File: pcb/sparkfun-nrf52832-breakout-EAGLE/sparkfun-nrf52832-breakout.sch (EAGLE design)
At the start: 72 parts, among them J1 DNP, Q1 2.5A/30V, U1 ESP8266, U2 MCP73831, U3 AT25SF041-SOIC8, U4 AP2112K-3.3V, U5 DNP, U6 DNP, U7 DNP, Y1 26MHz

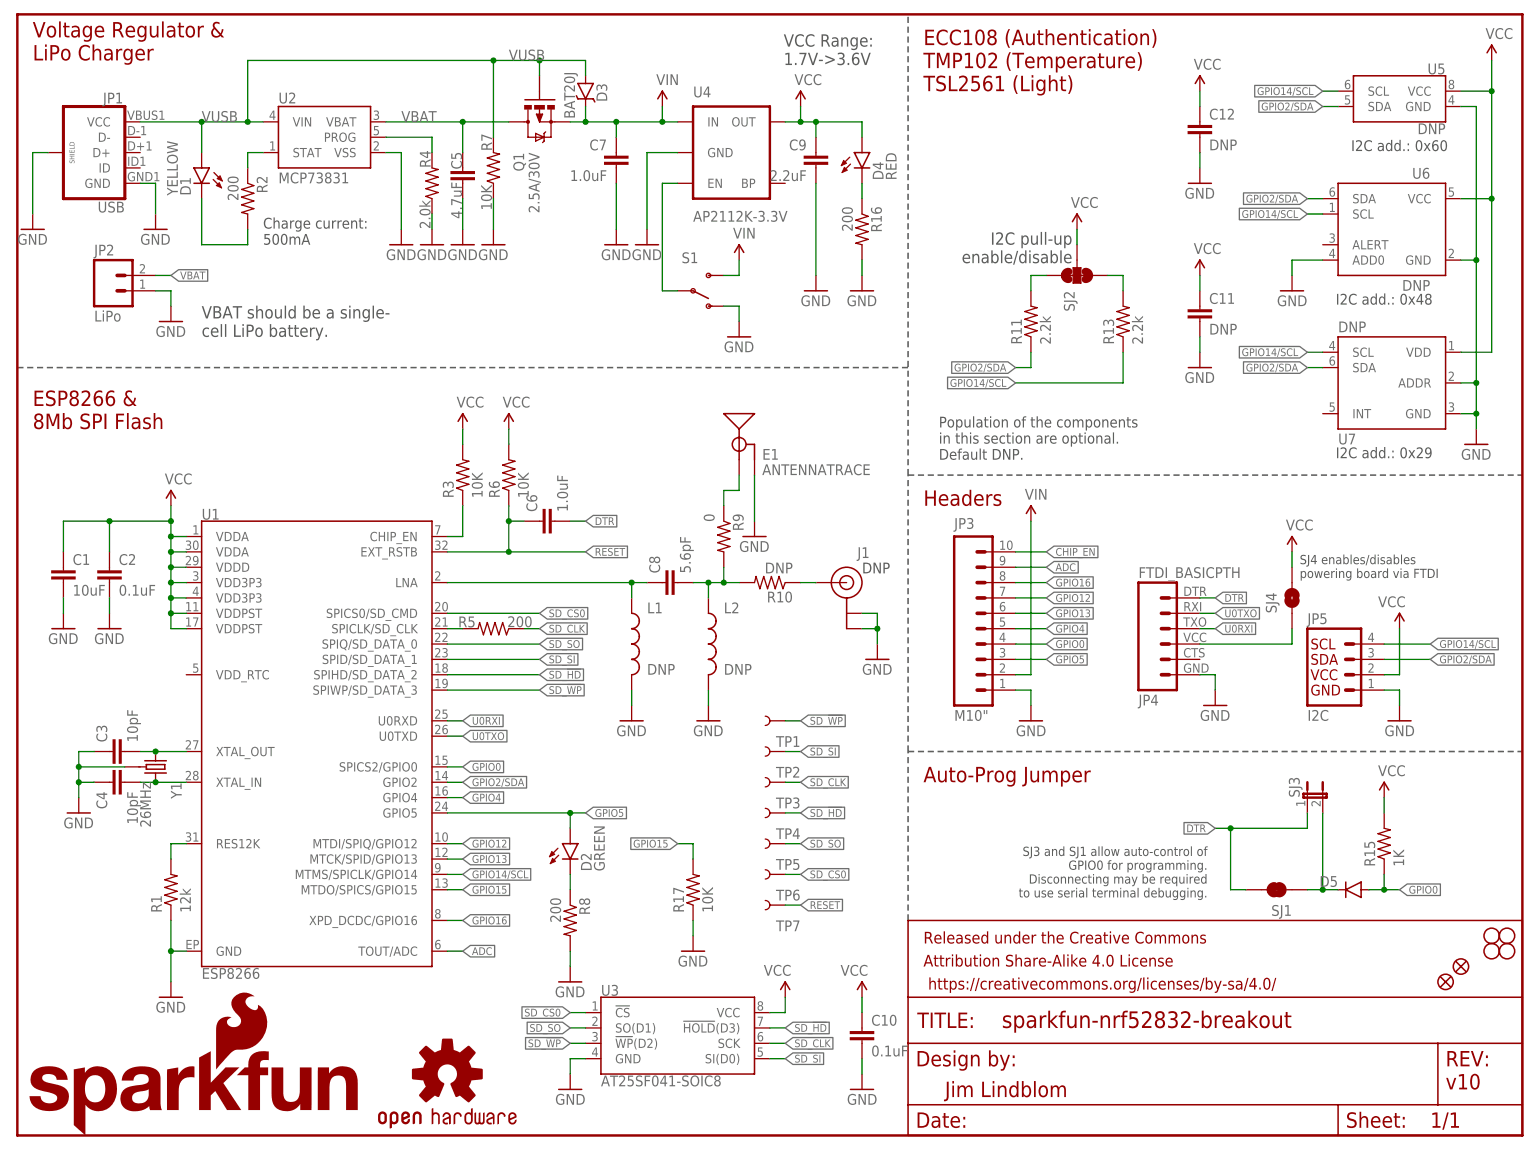
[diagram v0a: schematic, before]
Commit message: found antenna
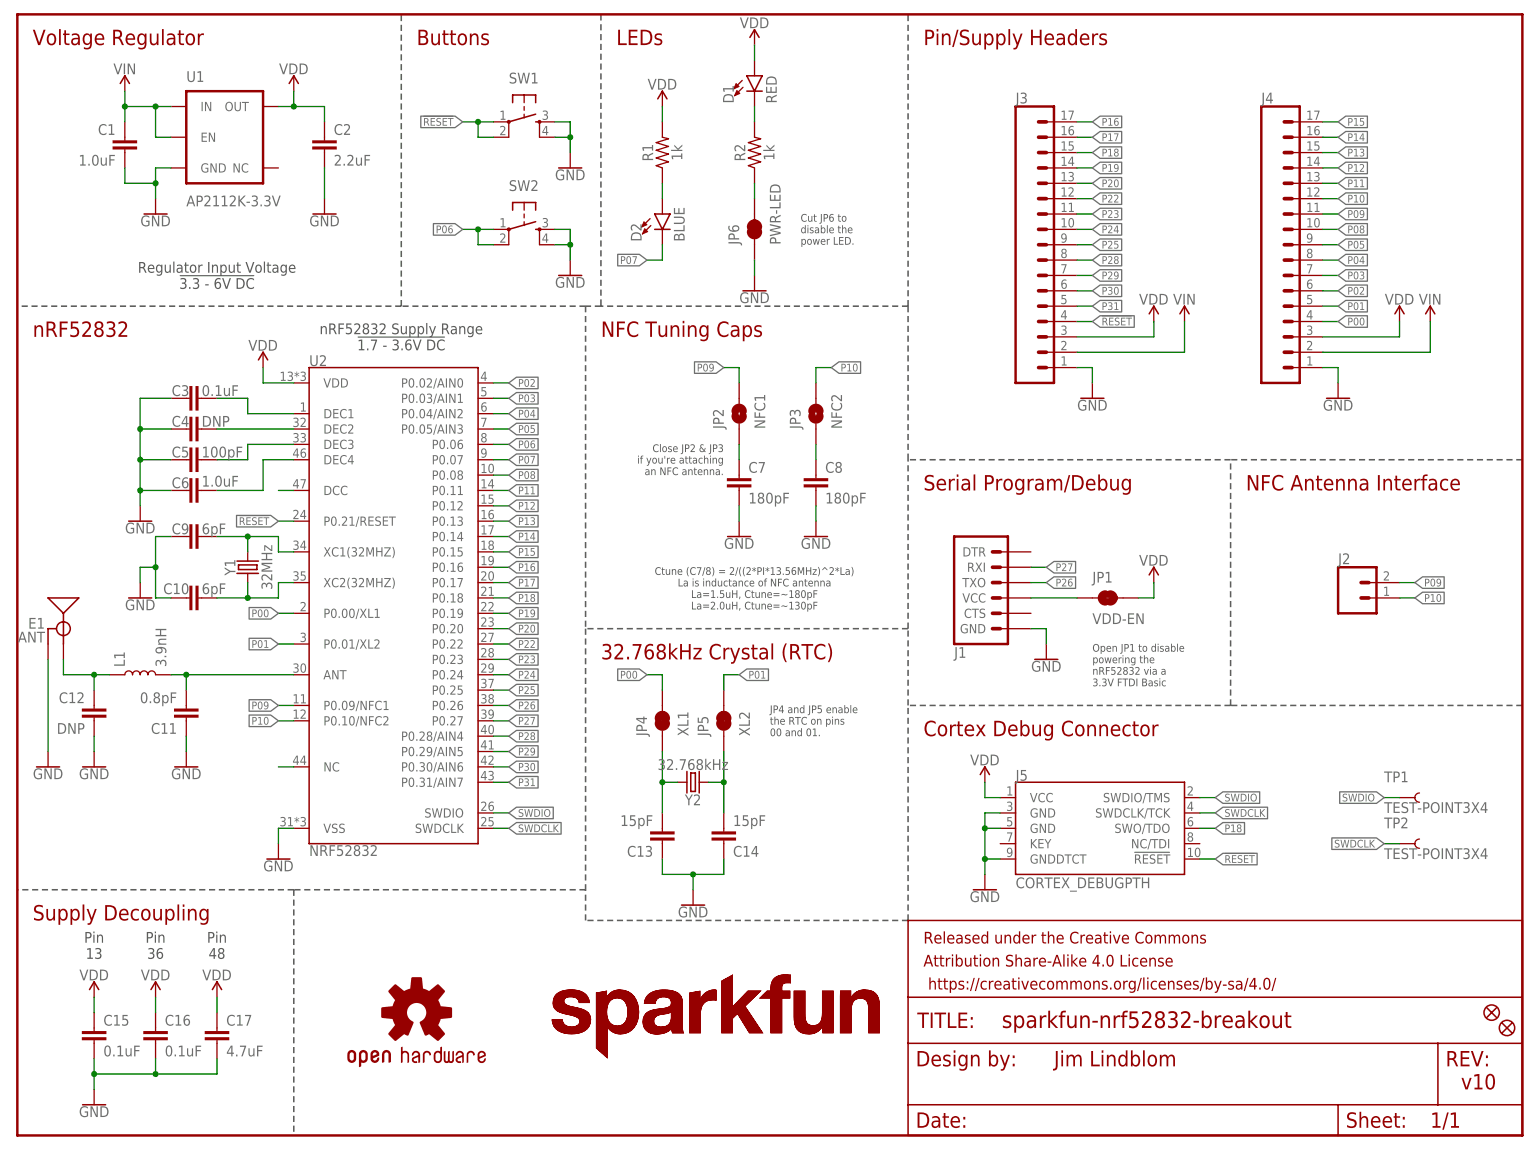
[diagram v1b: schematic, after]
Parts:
- removed D3: BAT20J, SparkFun-DiscreteSemi:DIODE-SCHOTTKY-BAT20J
- removed D4: RED, SparkFun-LED:LED-RED0603
- removed D5: (no value), SparkFun-DiscreteSemi:DIODEBAS16
- removed FID1, FID2: FIDUCIAL1X2, SparkFun-Aesthetics:FIDUCIAL1X2
- removed L2: DNP, SparkFun-Passives:INDUCTOR0603
- removed LOGO4: OSHW-LOGOS, SparkFun-Aesthetics:OSHW-LOGOS
- removed Q1: 2.5A/30V, SparkFun-DiscreteSemi:MOSFET-PCHANNELDMG2307L
- removed R10: DNP, SparkFun-Passives:RESISTOR0603-RES
- removed R11, R13: 2.2k, SparkFun-Resistors:2.2KOHM1/10W1%(0603)
- removed R15: 1K, SparkFun-Resistors:1KOHM1/10W1%(0603)
- removed R16, R5, R8: 200, SparkFun-Resistors:200OHM1/10W1%(0603)
- removed R17, R3, R6, R7: 10K, SparkFun-Resistors:10KOHM1/10W1%(0603)0603
- removed R4: 2.0k, SparkFun-Resistors:2.0KOHM1/10W5%(0603)
- removed R9: 0, SparkFun-Resistors:0OHM1/10W5%(0603)
- removed S1: (no value), SparkFun-Electromechanical:SWITCH-SPDT-SMD-A
- removed SJ1: JUMPER-PAD-2-NC_BY_TRACE, SparkFun-Passives:JUMPER-PAD-2-NC_BY_TRACE
- removed SJ2: (no value), SparkFun-Passives:JUMPER-PAD-3-NC_BY_TRACE
- removed SJ3: JUMPER-PTH-2-NC, SparkFun-Passives:JUMPER-PTH-2-NC
- removed SJ4: JUMPER-PAD-2-NOYES_SILK, SparkFun-Passives:JUMPER-PAD-2-NOYES_SILK
- removed STANDOFF1, STANDOFF2, STANDOFF3, STANDOFF4: STAND-OFF, SparkFun-Electromechanical:STAND-OFF
- removed TP3, TP4, TP5, TP6, TP7: TEST-POINT3X5, SparkFun-Passives:TEST-POINT3X5
- removed U3: AT25SF041-SOIC8, esp8266-development-board:AT25SF041-SOIC8
- removed U4: AP2112K-3.3V, SparkFun-PowerIC:V_REG_LDOSMD
- removed U5: DNP, esp8266-development-board:ATECC108-MAHDA
- removed U6: DNP, SparkFun-Sensors:TMP1021:1
- removed U7: DNP, esp8266-development-board:TSL2561FN
- added C13, C14: 15pF, SparkFun-Capacitors:15PF-0402-50V-5%
- added C15, C16: 0.1uF, SparkFun-Capacitors:0.1UF-0402-16V-10%
- added C17: 4.7uF, SparkFun-Capacitors:4.7UF0603
- added FD1, FD2: FIDUCIALUFIDUCIAL, SparkFun-Aesthetics:FIDUCIALUFIDUCIAL
- added J2: (no value), SparkFun-Connectors:CONN_02PTH
- added J3, J4: (no value), SparkFun-Connectors:CONN_17
- added J5: CORTEX_DEBUGPTH, SparkFun-Connectors:CORTEX_DEBUGPTH
- added JP6: PWR-LED, SparkFun-Jumpers:JUMPER-PAD-2-NC_BY_TRACE
- added LOGO2: SFE_LOGO_NAME.1_INCH, SparkFun-Aesthetics:SFE_LOGO_NAME.1_INCH
- added SW1, SW2: (no value), SparkFun-Electromechanical:SWITCH_SPST_4_PINRECT
- added Y2: 32.768kHz, SparkFun-Clocks:CRYSTAL-32.768KHZSMD-3.2X1.5
- C1: value 10uF -> 1.0uF; device SparkFun-Capacitors:10UF-6.3V-20%(0603) -> SparkFun-Capacitors:1.0UF-0603-16V-10%
- C10: value 0.1uF -> 6pF; device SparkFun-Capacitors:0.1UF-25V(+80/-20%)(0603) -> nrf52832-breakout-temp:6PF-0402-50V-0.5%
- C11: value DNP -> 0.8pF; device SparkFun-Capacitors:0.1UF-25V(+80/-20%)(0603) -> nrf52832-breakout-temp:0.8PF-0402-50V-0.1PF
- C12: device SparkFun-Capacitors:0.1UF-25V(+80/-20%)(0603) -> SparkFun-Passives:CAP0402
- C2: value 0.1uF -> 2.2uF; device SparkFun-Capacitors:0.1UF-25V(+80/-20%)(0603) -> SparkFun-Capacitors:2.2UF-0603-10V-20%
- C3: value 10pF -> 0.1uF; device SparkFun-Capacitors:10PF-50V-5%(0603) -> SparkFun-Capacitors:0.1UF-0402-16V-10%
- C4: value 10pF -> DNP; device SparkFun-Capacitors:10PF-50V-5%(0603) -> SparkFun-Passives:CAP0402
- C5: value 4.7uF -> 100pF; device SparkFun-Capacitors:4.7UF-6.3V-10%(0603)0603 -> nrf52832-breakout-temp:100PF-0402-50V-5%
- C6: device SparkFun-Capacitors:1.0UF-16V-10%(0603) -> SparkFun-Capacitors:1.0UF-0402-16V-10%
- C7: value 1.0uF -> 180pF; device SparkFun-Capacitors:1.0UF-25V-+80/-20(0805) -> nrf52832-breakout-temp:180PF-0603-50V-5%
- C8: value 5.6pF -> 180pF; device SparkFun-Capacitors:CAP0603-CAP -> nrf52832-breakout-temp:180PF-0603-50V-5%
- C9: value 2.2uF -> 6pF; device SparkFun-Capacitors:2.2UF-10V-20%(0603) -> nrf52832-breakout-temp:6PF-0402-50V-0.5%
- D1: value YELLOW -> RED; device SparkFun-LED:LED-YELLOW0603 -> SparkFun-LED:LED-RED0603
- D2: value GREEN -> BLUE; device SparkFun-LED:LED-GREEN0603 -> SparkFun-LED:LED-BLUE0603
- E1: value ANTENNATRACE -> ANT; device esp8266-development-board:ANTENNATRACE -> SparkFun-RF:ANTENNA-GROUNDEDTRACE-15.2MM
- J1: value DNP -> (none); device SparkFun-Connectors:U.FL -> SparkFun-Connectors:ARDUINO_SERIAL_PROGRAMPTH
- JP1: value USB -> VDD-EN; device SparkFun-Connectors:USB_MICROB_PLUGCONN-11752 -> SparkFun-Jumpers:JUMPER-SMT_2_NC_TRACE_SILK
- JP2: value LiPo -> NFC1; device SparkFun-Connectors:M02JST-PTH-2 -> SparkFun-Jumpers:JUMPER-SMT_2_NO_SILK
- JP3: value M10" -> NFC2; device SparkFun-Connectors:M10" -> SparkFun-Jumpers:JUMPER-SMT_2_NO_SILK
- JP4: value FTDI_BASICPTH -> XL1; device SparkFun-Connectors:FTDI_BASICPTH -> SparkFun-Jumpers:JUMPER-PAD-2-NC_BY_TRACE
- JP5: value I2C -> XL2; device SparkFun-Connectors:I2C_STANDARD -> SparkFun-Jumpers:JUMPER-PAD-2-NC_BY_TRACE
- L1: value DNP -> 3.9nH; device SparkFun-Passives:INDUCTOR0603 -> nrf52832-breakout-temp:INDUCTOR-0402-3.9NH
- LOGO1: value SFE_LOGO_NAME.2_INCH -> OSHW-LOGOMINI; device SparkFun-Aesthetics:SFE_LOGO_NAME.2_INCH -> SparkFun-Aesthetics:OSHW-LOGOMINI
- LOGO3: value SFE_LOGO_FLAME.1_INCH -> SFE_LOGO_NAME.1_INCH; device SparkFun-Aesthetics:SFE_LOGO_FLAME.1_INCH -> SparkFun-Aesthetics:SFE_LOGO_NAME.1_INCH
- R1: value 12k -> 1k; device SparkFun-Resistors:12KOHM-1/10W-1%(0603) -> SparkFun-Resistors:1KOHM-0603-1/10W-1%
- R2: value 200 -> 1k; device SparkFun-Resistors:200OHM1/10W1%(0603) -> SparkFun-Resistors:1KOHM-0603-1/10W-1%
- TP1, TP2: value TEST-POINT3X5 -> TEST-POINT3X4; device SparkFun-Passives:TEST-POINT3X5 -> SparkFun-Connectors:TEST-POINT3X4
- U1: value ESP8266 -> AP2112K-3.3V; device esp8266-development-board:ESP8266 -> SparkFun-PowerIC:V_REG_AP2112K-3.3V
- U2: value MCP73831 -> NRF52832; device SparkFun-PowerIC:MCP73831 -> nrf52832-breakout-temp:NRF52832
- Y1: value 26MHz -> 32MHz; device things:CRYSTAL-GROUNDED3.2X2.5 -> nrf52832-breakout-temp:CRYSTAL-32MHZ-SMD-2.0X1.6MM; PROD_ID XTAL-12454 -> (none)
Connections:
- removed net ADC: JP3.9, U1.TOUT/ADC
- removed net CHIP_EN: JP3.10, R3.1, U1.CHIP_EN
- removed net DTR: C6.2, JP4.1, SJ1.2, SJ3.1
- removed net FTDI_VCC: JP4.4, SJ4.1
- removed net GPIO0: D5.A, JP3.4, R15.1, U1.SPICS2/GPIO0
- removed net GPIO12: JP3.7, U1.MTDI/SPIQ/GPIO12
- removed net GPIO13: JP3.6, U1.MTCK/SPID/GPIO13
- removed net GPIO14/SCL: JP5.4, R13.1, U1.MTMS/SPICLK/GPIO14, U5.SCL, U6.SCL, U7.SCL
- removed net GPIO15: R17.2, U1.MTDO/SPICS/GPIO15
- removed net GPIO16: JP3.8, U1.XPD_DCDC/GPIO16
- removed net GPIO2/SDA: JP5.3, R11.1, U1.GPIO2, U5.SDA, U6.SDA, U7.SDA
- removed net GPIO4: JP3.5, U1.GPIO4
- removed net GPIO5: D2.A, JP3.3, U1.GPIO5
- removed net LNA: C8.1, L1.1, U1.LNA
- removed net N$10: R13.2, SJ2.3
- removed net N$18: R2.1, U2.STAT
- removed net N$2: C4.2, U1.XTAL_IN, Y1.2
- removed net N$5: C8.2, L2.1, R10.2, R9.2
- removed net N$6: R5.2, U1.SPICLK/SD_CLK
- removed net N$7: D5.C, SJ1.1, SJ3.2
- removed net N$9: R11.2, SJ2.1
- removed net RESET: C6.1, R6.1, TP7.1, U1.EXT_RSTB
- removed net SD_!HD!: TP4.1, U1.SPIHD/SD_DATA_2, U3.!HOLD!(D3)
- removed net SD_!WP!: TP1.1, U1.SPIWP/SD_DATA_3, U3.!WP!(D2)
- removed net SD_CLK: R5.1, TP3.1, U3.SCK
- removed net SD_CS0: TP6.1, U1.SPICS0/SD_CMD, U3.!CS!
- removed net SD_SI: TP2.1, U1.SPID/SD_DATA_1, U3.SI(D0)
- removed net SD_SO: TP5.1, U1.SPIQ/SD_DATA_0, U3.SO(D1)
- removed net TRACE_ANT: E1.SIGNAL, R9.1
- removed net U0RXI: JP4.3, U1.U0RXD
- removed net U0TXO: JP4.2, U1.U0TXD
- removed net VBAT: C5.1, JP2.2, Q1.D, U2.VBAT
- removed net VCC: C1.1, C10.1, C11.1, C12.1, C2.1, C9.1, D4.A, JP5.2, R15.2, R3.2, R6.2, SJ2.2, SJ4.2, U1.VDD3P3@3, U1.VDD3P3@4, U1.VDDA@1, U1.VDDA@30, U1.VDDD, U1.VDDPST@11, U1.VDDPST@17, U3.VCC, U4.OUT, U5.VCC, U6.VCC, U7.VDD
- removed net VUSB: D1.A, D3.A, JP1.VCC, Q1.G, R7.2, U2.VIN
- new net !RESET!: J3.4, J5.!RESET, SW1.1, SW1.2, U2.P0.21/RESET
- new net DCC: U2.DCC
- new net DEC1: C3.2, U2.DEC1
- new net DEC2: C4.2, U2.DEC2
- new net DEC3: C5.2, U2.DEC3
- new net DEC4: C6.2, U2.DEC4
- new net NC: U2.NC
- new net NFC1: C7.1, JP2.1
- new net NFC2: C8.1, JP3.1
- new net P00: J4.4, JP4.2, U2.P0.00/XL1
- new net P01: J4.5, JP5.2, U2.P0.01/XL2
- new net P02: J4.6, U2.P0.02/AIN0
- new net P03: J4.7, U2.P0.03/AIN1
- new net P04: J4.8, U2.P0.04/AIN2
- new net P05: J4.9, U2.P0.05/AIN3
- new net P06: SW2.1, SW2.2, U2.P0.06
- new net P07: D2.C, U2.P0.07
- new net P08: J4.10, U2.P0.08
- new net P09: J2.2, J4.11, JP2.2, U2.P0.09/NFC1
- new net P10: J2.1, J4.12, JP3.2, U2.P0.10/NFC2
- new net P11: J4.13, U2.P0.11
- new net P12: J4.14, U2.P0.12
- new net P13: J4.15, U2.P0.13
- new net P14: J4.16, U2.P0.14
- new net P15: J4.17, U2.P0.15
- new net P16: J3.17, U2.P0.16
- new net P17: J3.16, U2.P0.17
- new net P18: J3.15, J5.SWO/TDO, U2.P0.18
- new net P19: J3.14, U2.P0.19
- new net P20: J3.13, U2.P0.20
- new net P22: J3.12, U2.P0.22
- new net P23: J3.11, U2.P0.23
- new net P24: J3.10, U2.P0.24
- new net P25: J3.9, U2.P0.25
- new net P26: J1.TXO, U2.P0.26
- new net P27: J1.RXI, U2.P0.27
- new net P28: J3.8, U2.P0.28/AIN4
- new net P29: J3.7, U2.P0.29/AIN5
- new net P30: J3.6, U2.P0.30/AIN6
- new net P31: J3.5, U2.P0.31/AIN7
- new net SWDCLK: J5.SWDCLK/TCK, TP2.1, U2.SWDCLK
- new net SWDIO: J5.SWDIO/TMS, TP1.1, U2.SWDIO
- new net VDD: C15.1, C16.1, C17.1, C2.1, D1.A, J3.3, J4.3, J5.VCC, JP1.2, R1.2, U1.OUT, U2.VDD
- new net XC1: C9.2, U2.XC1(32MHZ), Y1.2
- new net XC2: C10.1, U2.XC2(32MHZ), Y1.1
- net ANT: now also C11.2, L1.2, U2.ANT; no longer J1.SIGNAL, R10.1
- net GND: now also C11.1, C13.1, C14.1, C15.2, C16.2, C17.2, C5.1, C6.1, C8.2, C9.1, J1.GND, J3.1, J4.1, J5.GND@3, J5.GND@5, J5.GNDDTCT, JP6.1, SW1.3, SW1.4, SW2.3, SW2.4; no longer C11.2, C5.2, C9.2, J1.GND@0, J1.GND@1, JP1.GND, JP1.SHIELD, JP2.1, JP3.1, JP4.6, JP5.1, L1.2, L2.2, R1.1, R16.2, R17.1, R4.1, R7.1, R8.2, S1.O, U3.GND, U4.GND, U5.GND, U6.ADD0, U6.GND, U7.ADDR, U7.GND, Y1.GND
- net N$1: now also JP6.2, R2.1; no longer R1.2, U1.RES12K
- net N$11: now also C12.1, E1.SIGNAL, L1.1; no longer S1.P, U4.EN
- net N$14: now also J1.VCC, JP1.1; no longer R4.2, U2.PROG
- net N$15: now also D2.A, R1.1; no longer D2.C, R8.1
- net N$3: now also C13.2, JP4.1, Y2.2; no longer C3.2, U1.XTAL_OUT, Y1.1
- net N$4: now also C14.2, JP5.1, Y2.1; no longer D4.C, R16.1
- net VIN: now also C1.1, J3.2, J4.2, U1.EN, U1.IN; no longer C7.1, D3.C, JP3.2, Q1.S, S1.S, U4.IN
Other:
- note added: "32.768kHz Crystal (RTC)"
- note added: "Buttons"
- note added: "Close JP2 & JP3 if you're attaching an NFC antenna."
- note added: "Cortex Debug Connector"
- note added: "Ctune (C7/8) = 2/((2*PI*13.56MHz)^2*La) La is inductance of NFC antenna La=1.5uH, Ctune=~180pF La=2.0uH, Ctune=~130pF"
- note added: "Cut JP6 to disable the power LED."
- note added: "JP4 and JP5 enable the RTC on pins 00 and 01."
- note added: "LEDs"
- note added: "NFC Antenna Interface"
- note added: "NFC Tuning Caps"
- note added: "Open JP1 to disable powering the nRF52832 via a 3.3V FTDI Basic"
- note added: "Pin 13"
- note added: "Pin 36"
- note added: "Pin 48"
- note added: "Pin/Supply Headers"
- note added: "Regulator Input Voltage !3.3 - 6V DC!"
- note added: "Serial Program/Debug"
- note added: "Supply Decoupling"
- note added: "Voltage Regulator"
- note added: "nRF52832"
- note added: "nRF52832 Supply Range !1.7 - 3.6V DC!"
- note removed: "Auto-Prog Jumper"
- note removed: "Charge current: 500mA"
- note removed: "DNP"
- note removed: "ECC108 (Authentication) TMP102 (Temperature) TSL2561 (Light)"
- note removed: "ESP8266 & 8Mb SPI Flash"
- note removed: "Headers"
- note removed: "I2C add.: 0x29"
- note removed: "I2C add.: 0x48"
- note removed: "I2C add.: 0x60"
- note removed: "I2C pull-up enable/disable"
- note removed: "Population of the components in this section are optional. Default DNP."
- note removed: "SJ3 and SJ1 allow auto-control of GPIO0 for programming. Disconnecting may be required to use serial terminal debugging."
- note removed: "SJ4 enables/disables powering board via FTDI"
- note removed: "VBAT should be a single- cell LiPo battery."
- note removed: "VCC Range: 1.7V->3.6V"
- note removed: "Voltage Regulator & LiPo Charger"
- moved on the sheet: C1, C10, C11, C12, C2, C3, C4, C5, C6, C7, C8, C9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
